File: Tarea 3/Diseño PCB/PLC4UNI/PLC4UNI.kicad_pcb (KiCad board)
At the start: 2 copper layers, 2 parts, among them J2 Screw_Terminal_01x18

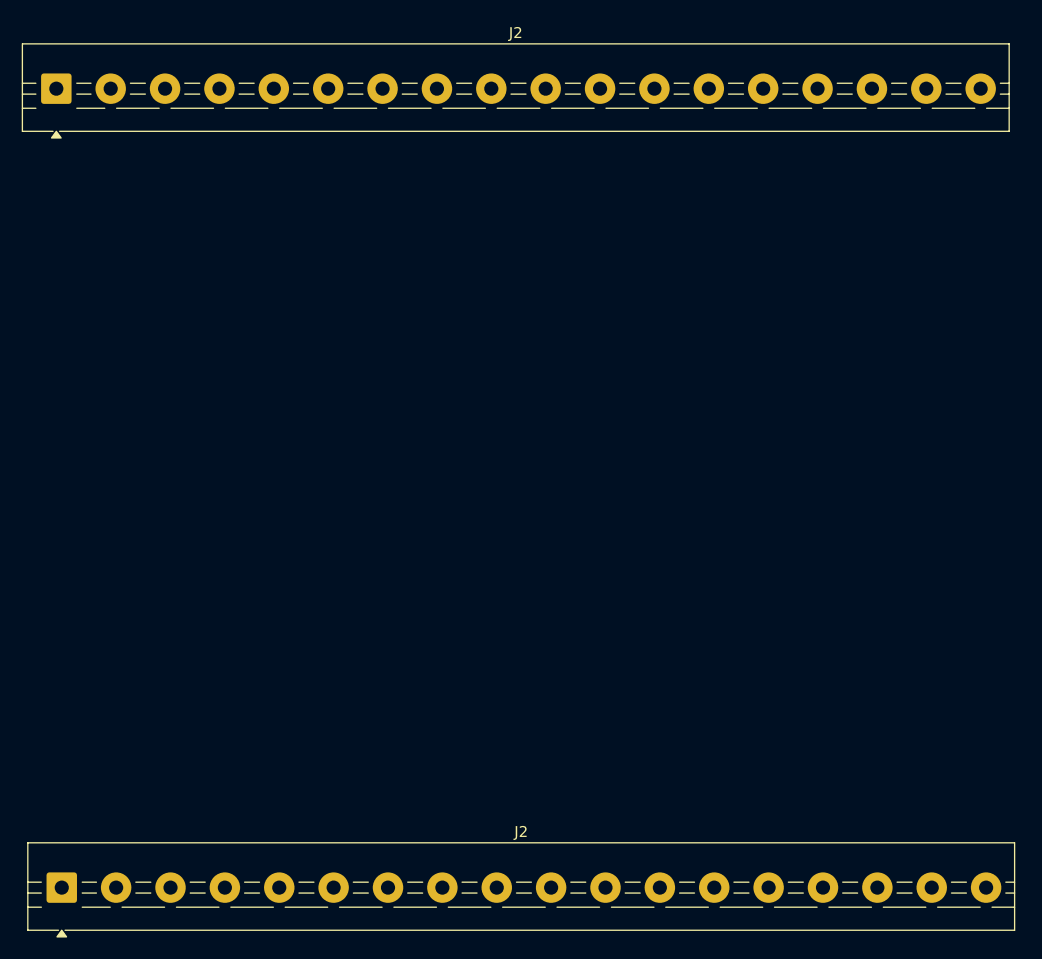
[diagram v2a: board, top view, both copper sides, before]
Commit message: Tarea  3
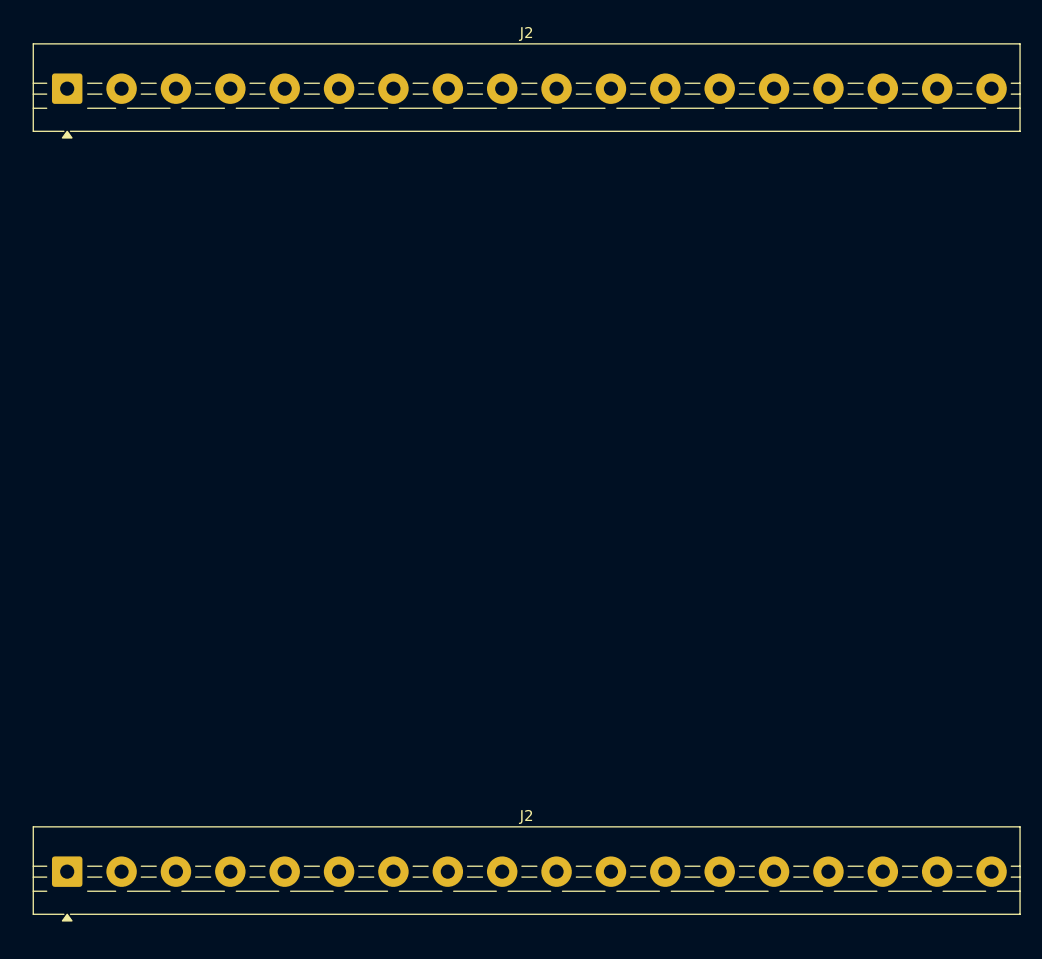
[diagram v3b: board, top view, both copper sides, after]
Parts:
- moved J2 1.55 mm to (71.0, 111.5)
- moved J2 1.00 mm to (71.0, 39.5)
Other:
- copper layers 2 -> 4
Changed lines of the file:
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@@
 	(layers
 		(0 "F.Cu" signal)
+		(4 "In1.Cu" signal)
+		(6 "In2.Cu" signal)
 		(2 "B.Cu" signal)
 		(9 "F.Adhes" user "F.Adhesive")
@@
 	)
 	(setup
+		(stackup
+			(layer "F.SilkS"
+				(type "Top Silk Screen")
+			)
+			(layer "F.Paste"
+				(type "Top Solder Paste")
+			)
+			(layer "F.Mask"
+				(type "Top Solder Mask")
+				(thickness 0.01)
+			)
+			(layer "F.Cu"
+				(type "copper")
+				(thickness 0.035)
+			)
+			(layer "dielectric 1"
+				(type "prepreg")
+				(thickness 0.1)
+				(material "FR4")
+				(epsilon_r 4.5)
+				(loss_tangent 0.02)
+			)
+			(layer "In1.Cu"
+				(type "copper")
+				(thickness 0.035)
+			)
+			(layer "dielectric 2"
+				(type "core")
+				(thickness 1.24)
+				(material "FR4")
+				(epsilon_r 4.5)
+				(loss_tangent 0.02)
+			)
+			(layer "In2.Cu"
+				(type "copper")
+				(thickness 0.035)
+			)
+			(layer "dielectric 3"
+				(type "prepreg")
+				(thickness 0.1)
+				(material "FR4")
+				(epsilon_r 4.5)
+				(loss_tangent 0.02)
+			)
+			(layer "B.Cu"
+				(type "copper")
+				(thickness 0.035)
+			)
+			(layer "B.Mask"
+				(type "Bottom Solder Mask")
+				(thickness 0.01)
+			)
+			(layer "B.Paste"
+				(type "Bottom Solder Paste")
+			)
+			(layer "B.SilkS"
+				(type "Bottom Silk Screen")
+			)
+			(copper_finish "None")
+			(dielectric_constraints no)
+		)
 		(pad_to_mask_clearance 0)
 		(allow_soldermask_bridges_in_footprints no)
 		(tenting front back)
+		(grid_origin 63 115.5)
 		(pcbplotparams
 			(layerselection 0x00000000_00000000_55555555_5755f5ff)
@@
 	(footprint "TerminalBlock:TerminalBlock_MaiXu_MX126-5.0-18P_1x18_P5.00mm"
 		(layer "F.Cu")
-		(at 70.5 112.9675)
+		(at 71 111.5)
 		(descr "terminal block MaiXu MX126-5.0-18P, 18 pins, pitch 5mm, size 90.5x7.8mm, drill diameter 1.3mm, pad diameter 2.8mm, https://www.lcsc.com/datasheet/lcsc_datasheet_2309150913_MAX-MX126-5-0-03P-GN01-Cu-S-A_C5188435.pdf, script-generated using https://gitlab.com/kicad/libraries/kicad-footprint-generator/-/tree/master/scripts/TerminalBlock_MaiXu")
 		(tags "THT terminal block MaiXu MX126-5.0-18P pitch 5mm size 90.5x7.8mm drill 1.3mm pad 2.8mm")
@@
 	(footprint "TerminalBlock:TerminalBlock_MaiXu_MX126-5.0-18P_1x18_P5.00mm"
 		(layer "F.Cu")
-		(at 70 39.5)
+		(at 71 39.5)
 		(descr "terminal block MaiXu MX126-5.0-18P, 18 pins, pitch 5mm, size 90.5x7.8mm, drill diameter 1.3mm, pad diameter 2.8mm, https://www.lcsc.com/datasheet/lcsc_datasheet_2309150913_MAX-MX126-5-0-03P-GN01-Cu-S-A_C5188435.pdf, script-generated using https://gitlab.com/kicad/libraries/kicad-footprint-generator/-/tree/master/scripts/TerminalBlock_MaiXu")
 		(tags "THT terminal block MaiXu MX126-5.0-18P pitch 5mm size 90.5x7.8mm drill 1.3mm pad 2.8mm")
@@
 	)
 	(gr_line
-		(start 62.895476 81.1)
-		(end 62.895476 115.682919)
+		(start 63 80.917081)
+		(end 63 115.5)
 		(stroke
 			(width 0.2)
@@
 	)
 	(gr_line
-		(start 62.895476 115.682919)
-		(end 162.822014 115.682919)
+		(start 63 115.5)
+		(end 162.926538 115.5)
 		(stroke
 			(width 0.2)
